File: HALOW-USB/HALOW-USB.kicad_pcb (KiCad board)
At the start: 2 copper layers, 15 x 32 mm, 12 parts, among them U1 TLV75533PDBVR, U2 GT-USB-7010ASV

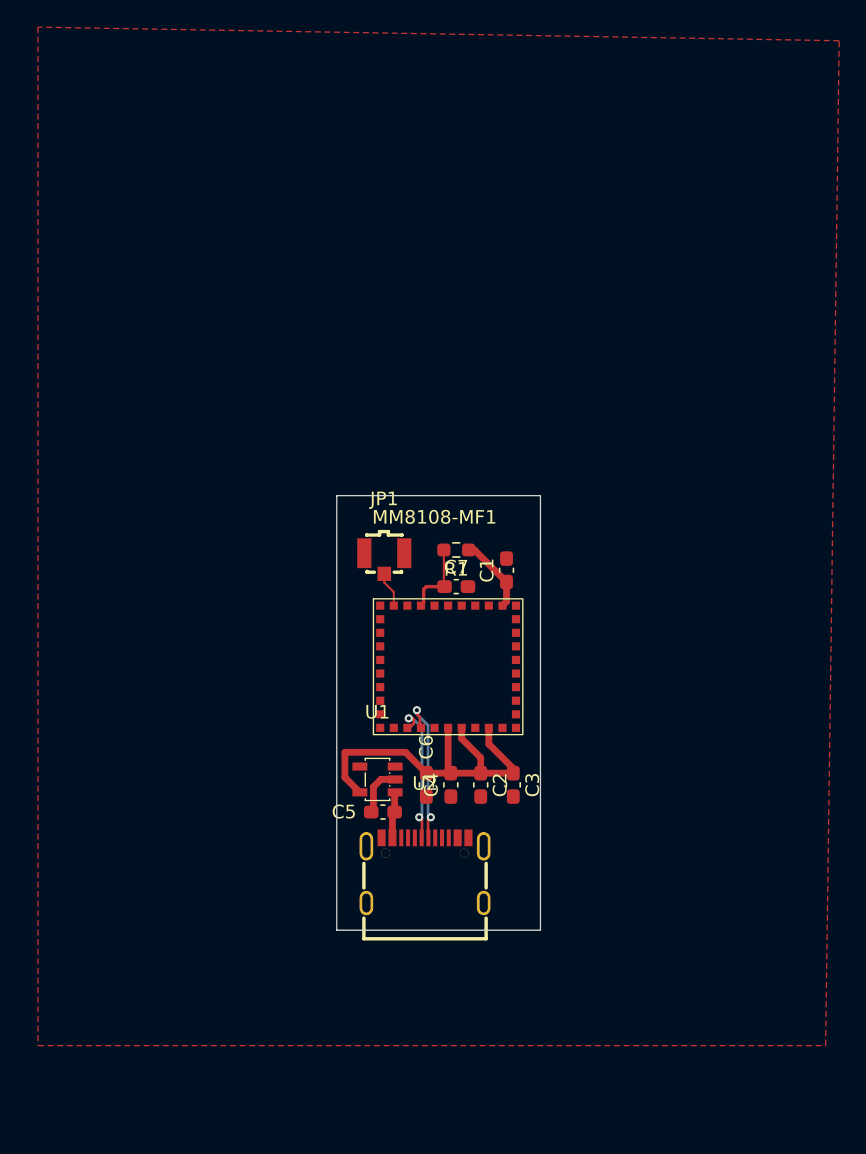
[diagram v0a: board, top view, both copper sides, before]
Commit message: trace work
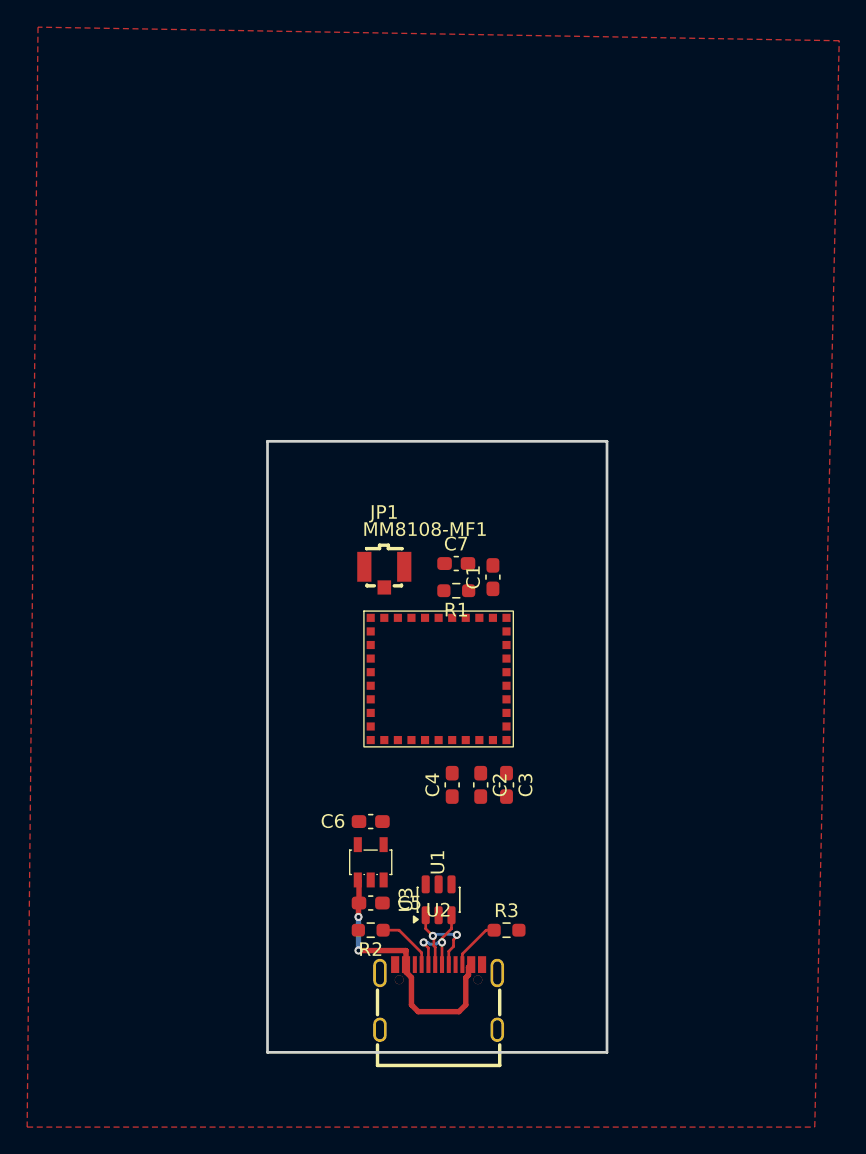
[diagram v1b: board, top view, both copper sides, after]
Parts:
- added R2: 5k1, Resistor_SMD:R_0603_1608Metric_Pad0.98x0.95mm_HandSolder, F.Cu at (118.5, 103.5)
- added R3: 5k1, Resistor_SMD:R_0603_1608Metric_Pad0.98x0.95mm_HandSolder, F.Cu at (128.5, 103.5)
- added U3: USBLC6-2SC6, Package_TO_SOT_SMD:SOT-23-6, F.Cu at (123.5, 101.3)
- moved U2 9.39 mm to (123.5, 108.4)
- moved C5 6.76 mm to (118.5, 101.5), turned to 0 degrees
- moved U1 6.12 mm to (118.5, 98.5), turned to -90 degrees
- moved C6 4.91 mm to (118.5, 95.5), turned to 0 degrees
- moved R1 3.00 mm to (124.8, 78.5)
- moved C7 1.70 mm to (124.8, 76.5)
- moved MM8108-MF1 1.14 mm to (118.5, 80.5)
- moved C1 1.12 mm to (127.5, 77.5)
- moved JP1 1.00 mm to (119.5, 77.5)
- moved C3 0.50 mm to (128.5, 92.8)
- moved C4 0.10 mm to (124.5, 92.8)
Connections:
- net /5v_in renamed +5V
- MM8108-MF1 pad 27: USB_D- -> /USB/USB D-
- MM8108-MF1 pad 28: USB_D+ -> /USB/USB_D+
- U2 pad A5: unconnected-(U2-CC1-PadA5) -> Net-(U2-CC1)
- U2 pad A6: USB_D+ -> /USB/PRE D+
- U2 pad A7: USB_D- -> /USB/PRE D-
- U2 pad B5: unconnected-(U2-CC2-PadB5) -> Net-(U2-CC2)
- U2 pad B6: USB_D+ -> /USB/PRE D+
- U2 pad B7: USB_D- -> /USB/PRE D-
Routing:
- net +3.3V: track 34.2 -> 0.00 mm
- net +5V: track 3.43 -> 20.5 mm, vias 0 -> 2
- net USB_D-: track 11.3 -> 0.00 mm, vias 2 -> 0
- net USB_D+: track 10.9 -> 0.00 mm, vias 2 -> 0
- net /USB/PRE D+: track 0.00 -> 8.26 mm, vias 0 -> 2
- net /USB/PRE D-: track 0.00 -> 7.15 mm, vias 0 -> 2
- net /reset: track 5.76 -> 0.00 mm
- net Net-(U2-CC1): track 0.00 -> 4.40 mm
- net Net-(U2-CC2): track 0.00 -> 3.84 mm
- net GND: track 3.75 -> 0.00 mm
- net /RF_OUT: track 2.69 -> 0.00 mm
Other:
- board size 15 x 32 mm -> 25 x 45 mm

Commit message: mfg files added
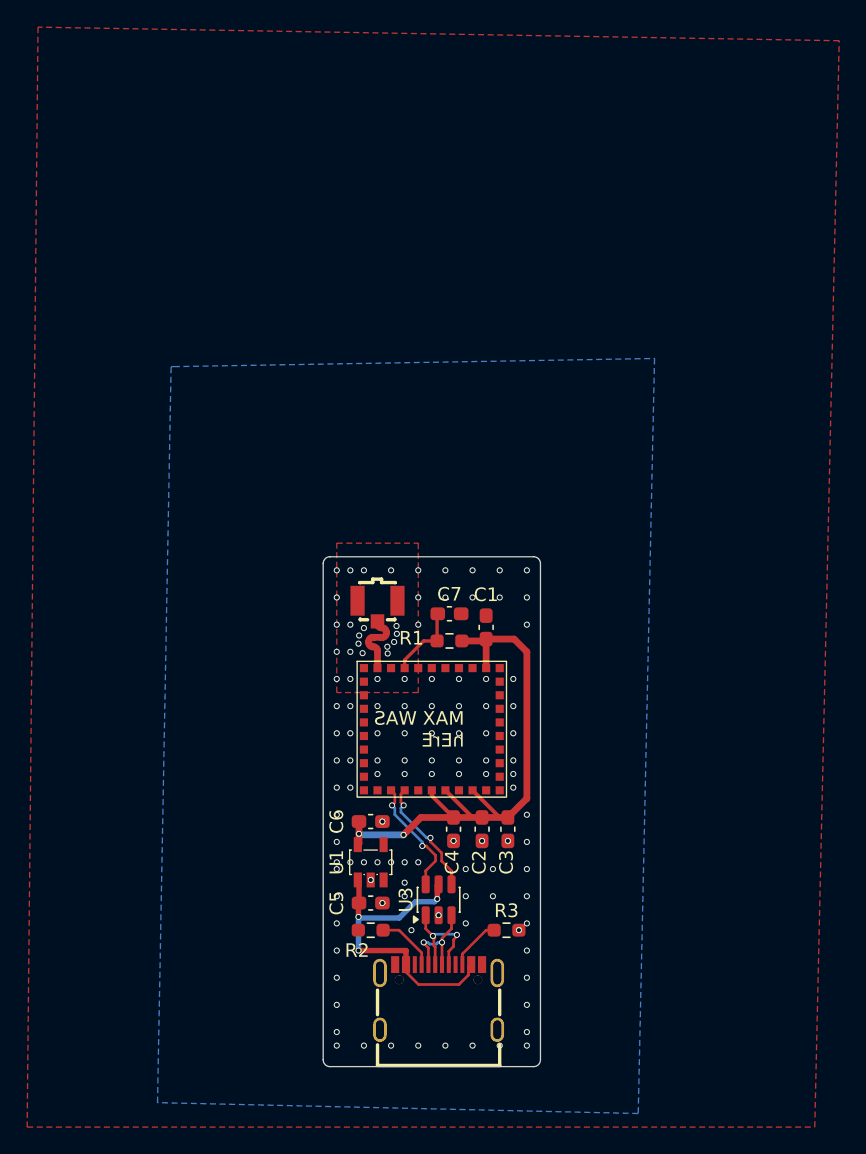
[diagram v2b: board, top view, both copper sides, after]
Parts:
- added G***: LOGO, LOGO, B.Cu at (123.2, 95.0)
- moved C1 3.73 mm to (127.0, 81.2)
- moved C7 3.73 mm to (124.3, 80.2)
- moved MM8108-MF1 3.73 mm to (118.0, 84.2)
- moved R1 3.73 mm to (124.3, 82.2)
- moved C2 3.26 mm to (126.7, 96.1)
- moved C3 3.26 mm to (128.6, 96.1)
- moved C4 3.26 mm to (124.6, 96.1)
- moved JP1 2.55 mm to (119.0, 80.0)
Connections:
- net /USB/USB D- renamed /D -
- net /USB/USB_D+ renamed /D +
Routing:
- net +3.3V: track 0.00 -> 43.0 mm, vias 0 -> 2
- net /D +: track 0.00 -> 8.91 mm, vias 0 -> 2
- net /D -: track 0.00 -> 8.91 mm, vias 0 -> 2
- net /reset: track 0.00 -> 5.59 mm
- net /RF_OUT: track 0.00 -> 5.26 mm
- net +5V: track 20.5 -> 24.0 mm, vias 2 -> 3
- net GND: vias 0 -> 120
- added copper zone on B.Cu, net GND
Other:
- board size 25 x 45 mm -> 16 x 37.5 mm
- board text added: "MAX WAS hErE"
- board text added: "R01. HOTPINK"
